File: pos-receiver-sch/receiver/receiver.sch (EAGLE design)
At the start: 17 parts, among them IC1 AD8599R

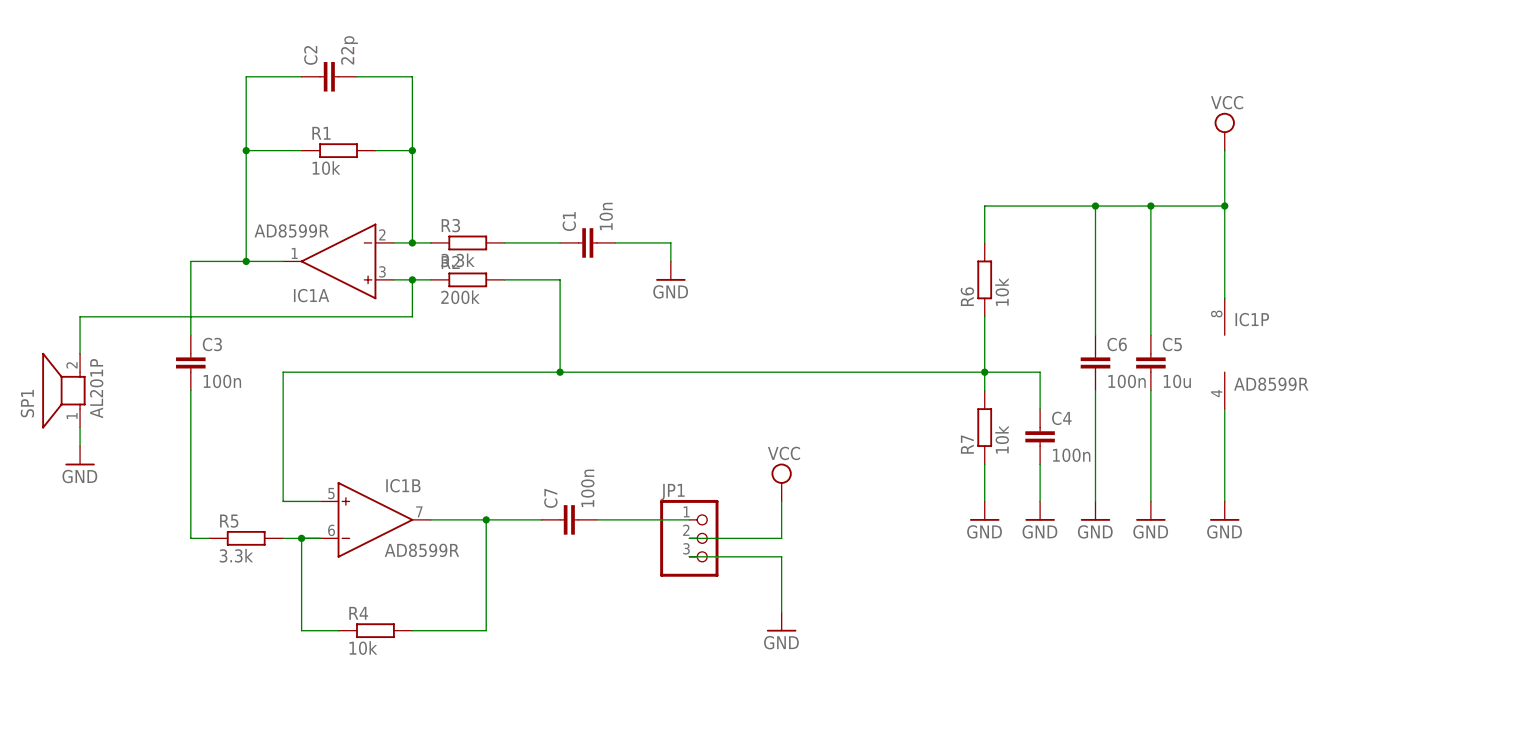
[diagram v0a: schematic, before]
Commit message: receiver-sch ver: 0.2
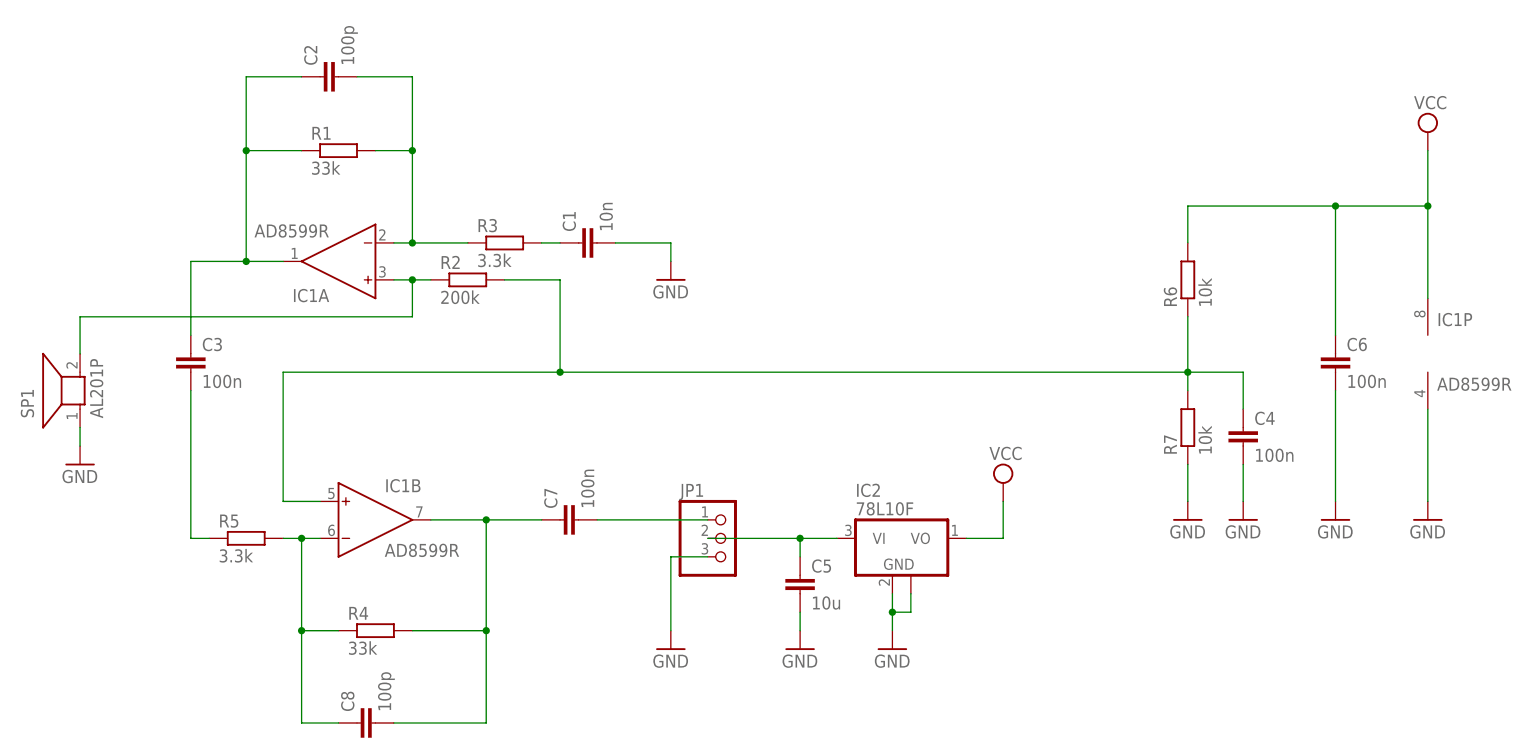
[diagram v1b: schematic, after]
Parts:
- added C8: 100p, resistor:C-EUC1206K
- added IC2: 78L10F, linear:78L10F
- C2: value 22p -> 100p
- R1, R4: value 10k -> 33k
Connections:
- new net N$10: C5.1, IC2.VI, JP1.2
- net GND: now also IC2.GND, IC2.GND@1
- net N$4: now also C8.1
- net N$5: now also C8.2
- net VCC: now also IC2.VO; no longer C5.1, JP1.2
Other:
- moved on the sheet: C4, C5, C6, IC1P, JP1, R3, R6, R7

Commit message: charge amp
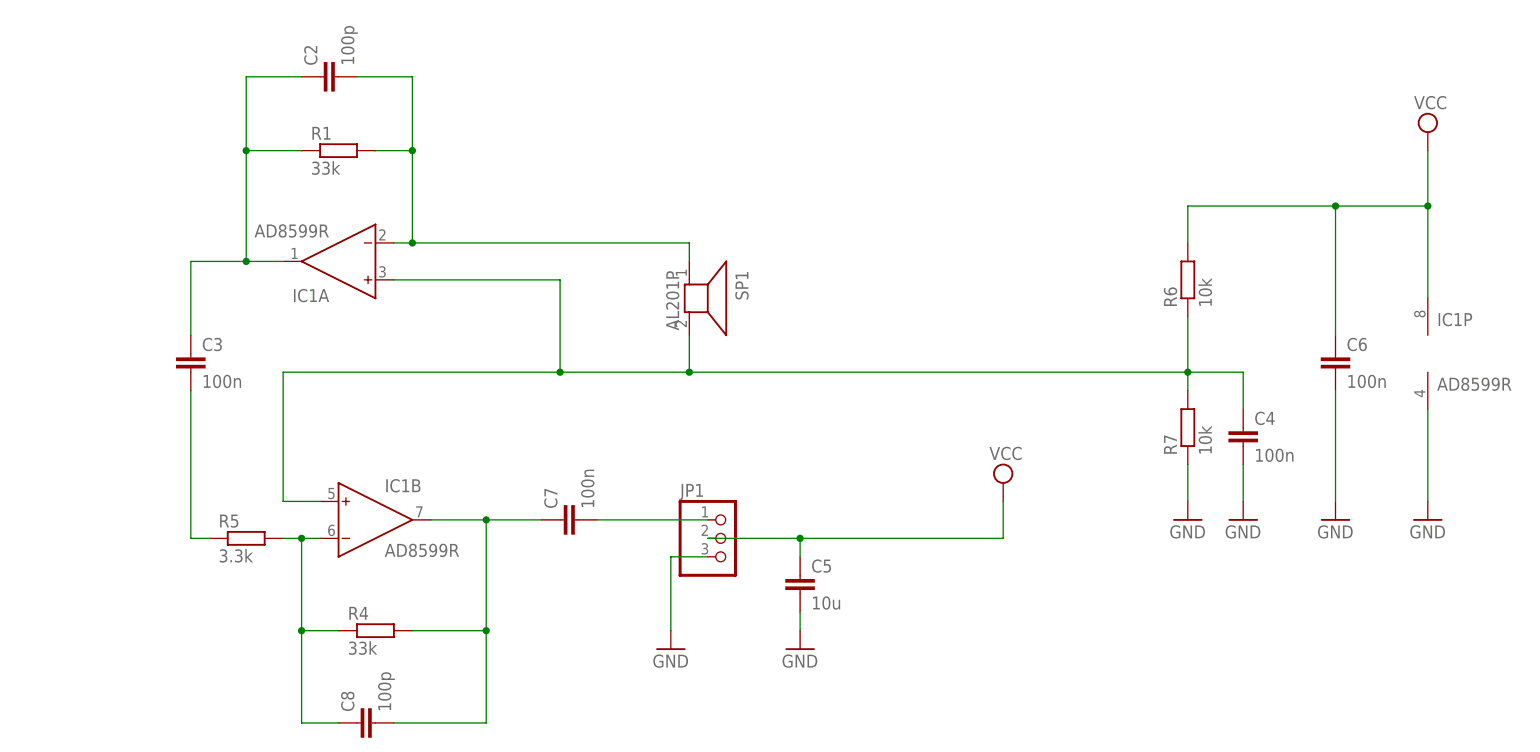
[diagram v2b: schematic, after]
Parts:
- removed C1: 10n, resistor:C-EUC1206K
- removed IC2: 78L10F, linear:78L10F
- removed R2: 200k, resistor:R-EU_R0805
- removed R3: 3.3k, resistor:R-EU_R0805
- C7: device resistor:C-EUC1206 -> resistor:C-EUC1206K
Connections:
- removed net N$10: C5.1, IC2.VI, JP1.2
- removed net N$2: C2.2, IC1A.IN-, R1.2, R3.1
- removed net N$7: IC1A.IN+, R2.1, SP1.2
- net GND: no longer C1.2, IC2.GND, IC2.GND@1, SP1.1
- net N$3: now also C2.2, IC1A.IN-, R1.2, SP1.1; no longer C1.1, R3.2
- net N$9: now also IC1A.IN+, SP1.2; no longer R2.2
- net VCC: now also C5.1, JP1.2; no longer IC2.VO
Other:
- moved on the sheet: SP1

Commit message: pcb
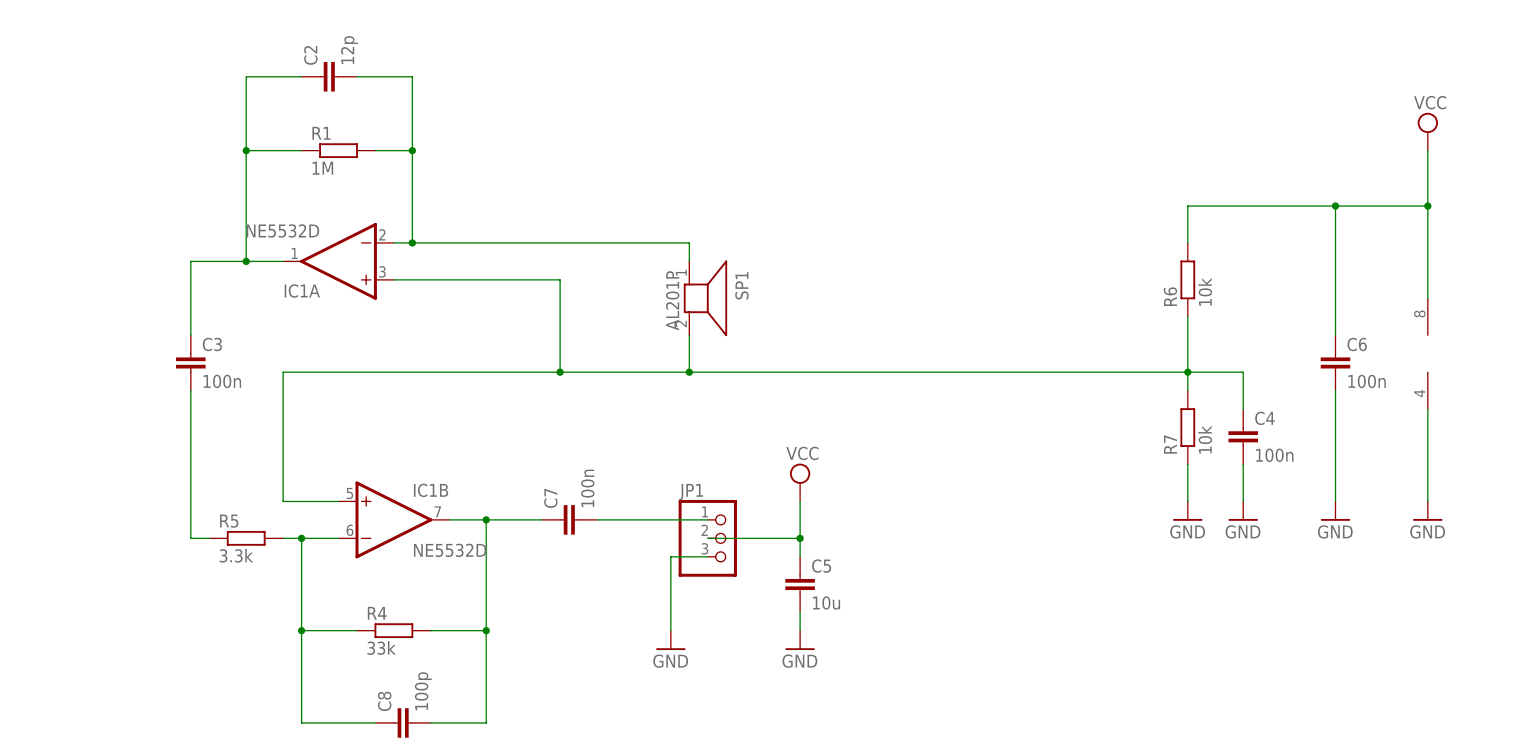
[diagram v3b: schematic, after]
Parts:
- C2: value 100p -> 12p; device resistor:C-EUC1206K -> resistor:C-EUC0805
- C3, C4, C5, C8: device resistor:C-EUC1206K -> resistor:C-EUC0805
- IC1: value AD8599R -> NE5532D; device analog-devices:AD8599R -> linear:NE5532D
- R1: value 33k -> 1M
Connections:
- net N$3: now also IC1A.-IN; no longer IC1A.IN-
- net N$4: now also IC1B.-IN; no longer IC1B.IN-
- net N$9: now also IC1A.+IN, IC1B.+IN; no longer IC1A.IN+, IC1B.IN+
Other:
- moved on the sheet: C8, IC1B, R4
